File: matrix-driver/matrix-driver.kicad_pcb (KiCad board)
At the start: 4 copper layers, 35 parts, among them IC1 SPX5205M5-L-3-3_TR, J1 Conn_01x09, J2 Conn_01x08, J3 Conn_01x27, J4 Conn_01x27, J5 Conn_01x08, U1 TPS562202, U2 LP5891MRRFR, U3 TPS562202

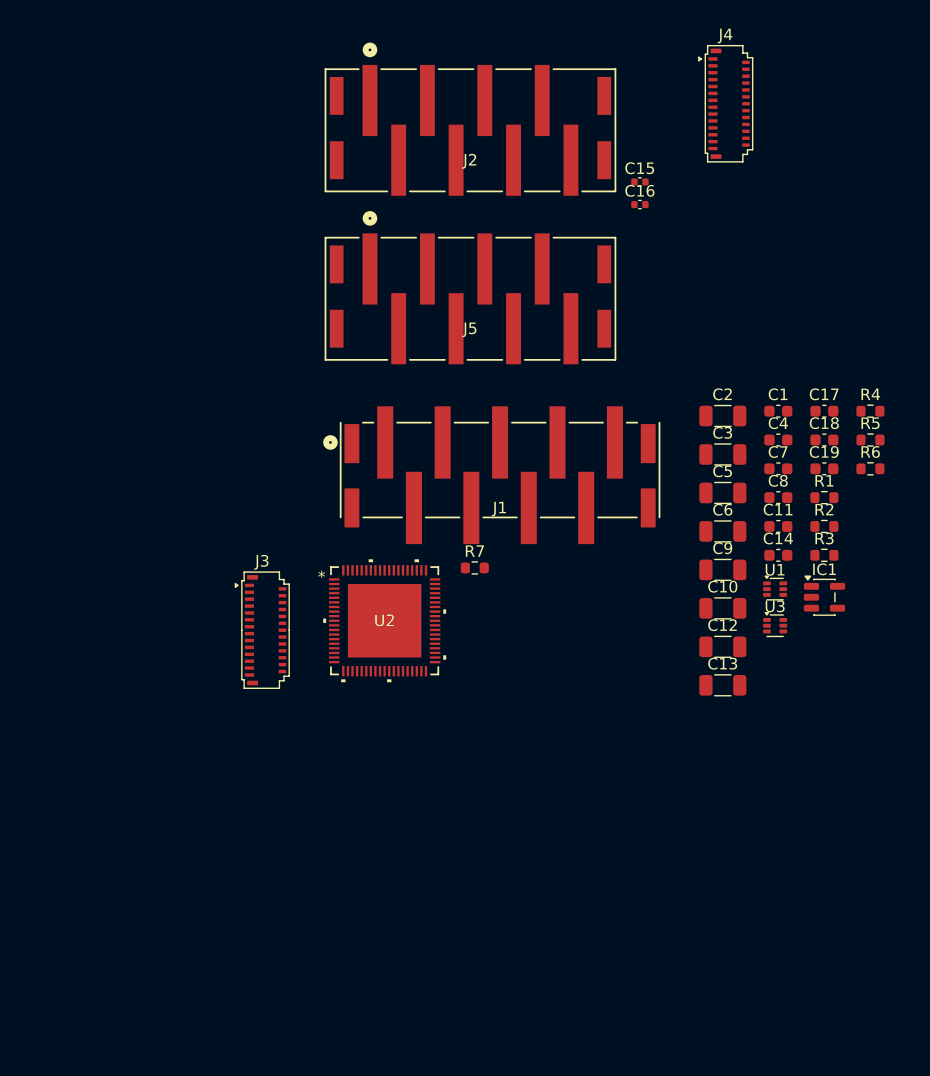
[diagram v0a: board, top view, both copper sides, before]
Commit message: added gerbers and finalized v1.0
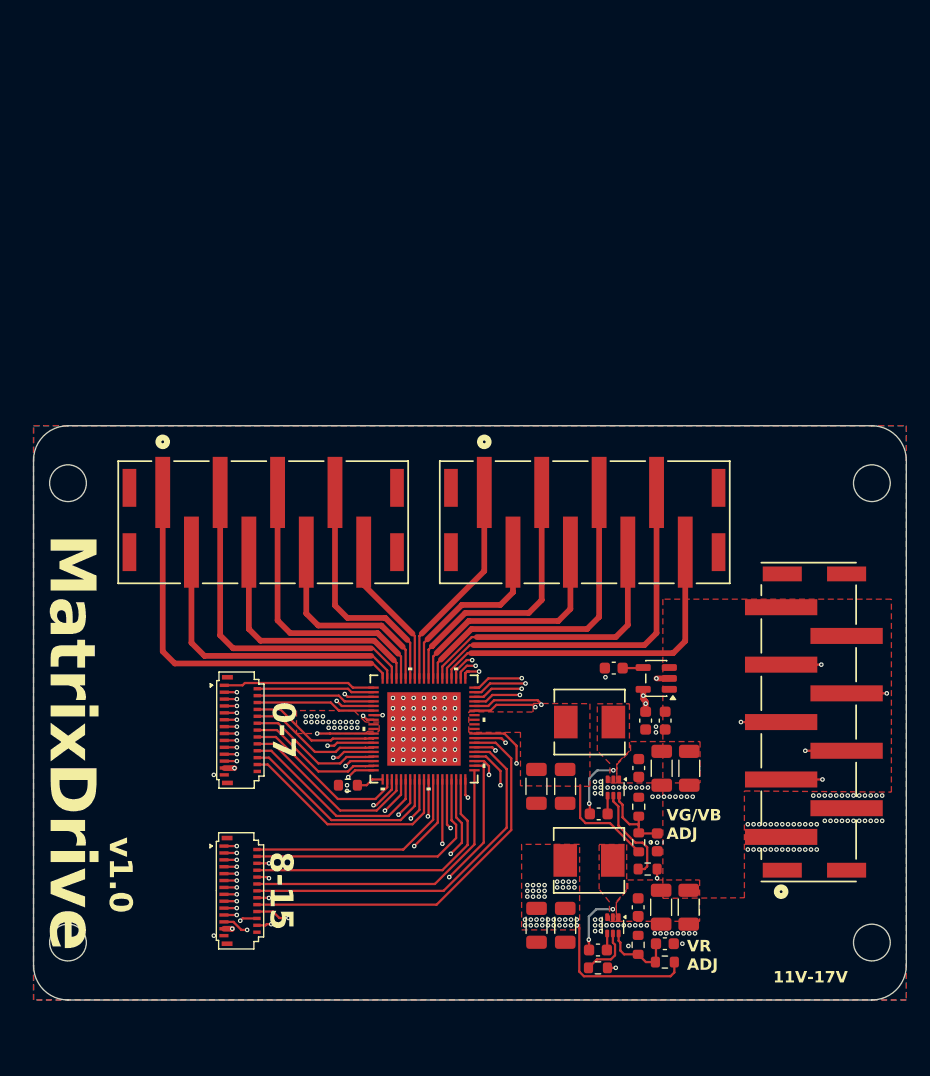
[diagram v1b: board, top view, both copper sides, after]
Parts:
- removed C15, C16: 0.1uF, Capacitor_SMD:C_0402_1005Metric
- added H1: MountingHole, MountingHole:MountingHole_3.2mm_M3_DIN965, F.Cu at (100.0, 98.0)
- added H2: MountingHole, MountingHole:MountingHole_3.2mm_M3_DIN965, F.Cu at (170.0, 98.0)
- added H3: MountingHole, MountingHole:MountingHole_3.2mm_M3_DIN965, F.Cu at (100.0, 138.0)
- added H4: MountingHole, MountingHole:MountingHole_3.2mm_M3_DIN965, F.Cu at (170.0, 138.0)
- added L1: 4.7uH, ETQ_P3M3R3KVP:IND_PCC-M0530M-LP_PAN, F.Cu at (145.4, 118.8)
- added L2: 3.3uH, ETQ_P3M3R3KVP:IND_PCC-M0530M-LP_PAN, F.Cu at (145.4, 130.8)
- C12, C13: value 22uF -> 33uF
- C14: value 10nF -> 10pF
- C7: value 10nF -> 22pF
- moved J4 80.7 mm to (115.0, 133.5)
- moved R4 54.0 mm to (146.2, 140.2), turned to 180 degrees
- moved R5 48.9 mm to (152.0, 139.7), turned to 180 degrees
- moved R6 46.1 mm to (149.7, 138.2), turned to 90 degrees
- moved C8 42.4 mm to (146.2, 138.7)
- moved J2 38.6 mm to (117.0, 101.4)
- moved C1 38.4 mm to (146.2, 126.8)
- moved R1 35.8 mm to (150.5, 131.6), turned to 180 degrees
- moved C11 35.3 mm to (149.7, 134.9), turned to -90 degrees
- moved C14 35.2 mm to (152.0, 138.1), turned to 180 degrees
- moved J1 34.7 mm to (164.5, 118.8), turned to 90 degrees
- moved C7 34.2 mm to (151.3, 129.3), turned to 90 degrees
- moved R2 31.9 mm to (149.7, 129.3), turned to 90 degrees
- moved C4 31.0 mm to (149.7, 122.8), turned to -90 degrees
- moved C2 30.8 mm to (154.1, 122.8), turned to -90 degrees
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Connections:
- C17 pad 1: Net-(IC1-EN) -> +12V
- IC1 pad 1: Net-(IC1-EN) -> +12V
- IC1 pad 3: Net-(IC1-EN) -> +12V
- J3 pad 25: +3.3V -> +3V3
- J4 pad 25: +3.3V -> +3V3
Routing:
- net +3V3: track 0.00 -> 61.5 mm, vias 0 -> 5
- net /R15: track 0.00 -> 54.8 mm, vias 0 -> 2
- net /G15: track 0.00 -> 52.2 mm, vias 0 -> 2
- net /B15: track 0.00 -> 47.5 mm, vias 0 -> 2
- net /B14: track 0.00 -> 46.8 mm, vias 0 -> 2
- net /R14: track 0.00 -> 45.9 mm, vias 0 -> 2
- net /G14: track 0.00 -> 45.8 mm, vias 0 -> 2
- net /2V8_EN: track 0.00 -> 42.6 mm, vias 0 -> 2
- net /G13: track 0.00 -> 40.0 mm, vias 0 -> 2
- net /SOUT: track 0.00 -> 39.1 mm, vias 0 -> 2
- net /SIN: track 0.00 -> 37.5 mm, vias 0 -> 2
- net /R13: track 0.00 -> 36.6 mm, vias 0 -> 2
- net /R12: track 0.00 -> 35.1 mm, vias 0 -> 2
- net /B12: track 0.00 -> 34.9 mm, vias 0 -> 2
- net /B13: track 0.00 -> 34.8 mm
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- added copper zone on F.Cu, net +12V
- added copper zone on F.Cu, net +2V8
- added copper zone on In2.Cu, net +2V8
- added copper zone on F.Cu, net +3V8
- added copper zone on B.Cu, net GND
- added copper zone on F.Cu, net GND
- added copper zone on In1.Cu, net GND
- added copper zone on In2.Cu, net GND
- added copper zone on F.Cu, net Net-(U1-SW)
- added copper zone on F.Cu, net Net-(U3-SW)
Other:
- board outline added: 76 x 50 mm
- board text added: "0-7"
- board text added: "11V-17V"
- board text added: "8-15"
- board text added: "MatrixDrive"
- board text added: "VG/VB ADJ"
- board text added: "VR ADJ"
- board text added: "v1.0"
